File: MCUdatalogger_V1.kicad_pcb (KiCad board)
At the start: 2 copper layers, 29 parts, among them J1 Conn_01x04_Pin, J2 Conn_01x04_Pin, J3 Conn_01x09_Pin, J4 Conn_02x03_Odd_Even, U1 24LC1025, U2 DS1337S+, U3 24LC1025, U4 ATMEGA328P-AU, Y1 32.768 KHz, Y2 16 MHz

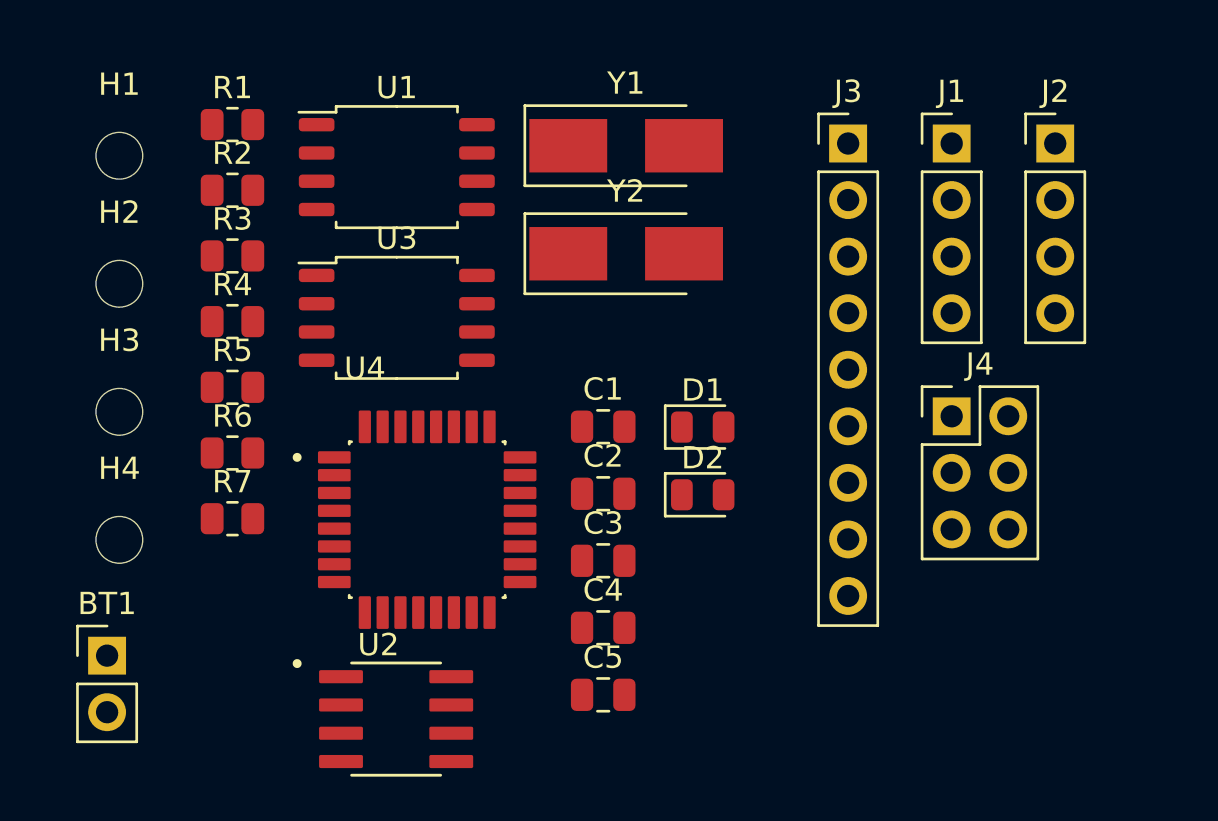
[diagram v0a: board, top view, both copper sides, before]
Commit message: Connections established
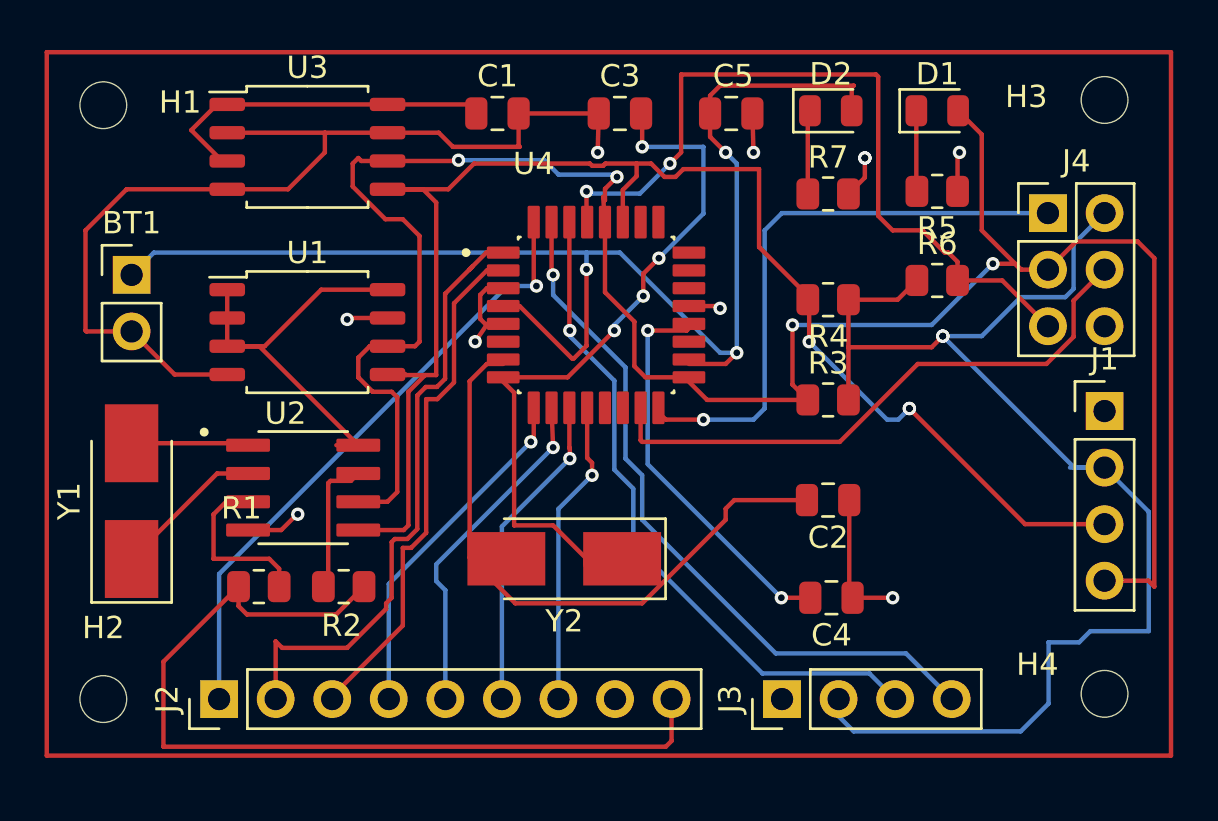
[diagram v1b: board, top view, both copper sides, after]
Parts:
- moved H3 46.4 mm to (123.7, 46.8)
- moved H4 44.8 mm to (123.7, 73.4)
- moved J2 37.7 mm to (83.9, 73.7), turned to 90 degrees
- moved R5 32.9 mm to (116.2, 50.9), turned to 180 degrees
- moved R6 32.6 mm to (116.2, 54.9)
- moved R7 30.5 mm to (111.3, 51.0)
- moved J3 27.8 mm to (109.2, 73.7), turned to 90 degrees
- moved R3 27.5 mm to (111.3, 60.2)
- moved Y1 27.3 mm to (80.0, 64.8), turned to 90 degrees
- moved R4 26.8 mm to (111.3, 55.7), turned to 180 degrees
- moved C5 26.7 mm to (106.9, 47.4)
- moved R1 20.8 mm to (85.7, 68.6)
- moved C3 20.1 mm to (101.9, 47.4)
- moved H2 18.7 mm to (78.7, 73.7)
- moved R2 18.5 mm to (89.5, 68.6), turned to 180 degrees
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- renumbered J3 to J2, J2 to J3
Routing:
- net /VCC: track 0.00 -> 137.1 mm, vias 0 -> 2
- net /SCK: track 0.00 -> 100.2 mm, vias 0 -> 4
- net /SDA: track 0.00 -> 68.1 mm, vias 0 -> 3
- net GND: track 0.00 -> 67.0 mm, vias 0 -> 10
- net Net-(BT1-+): track 0.00 -> 60.8 mm, vias 0 -> 3
- net /RESET: track 0.00 -> 35.5 mm, vias 0 -> 2
- net /TX: track 0.00 -> 32.1 mm, vias 0 -> 1
- net Net-(U4-PB7): track 0.00 -> 30.8 mm, vias 0 -> 4
- net /RX: track 0.00 -> 30.1 mm, vias 0 -> 1
- net /D2: track 0.00 -> 28.1 mm, vias 0 -> 1
- net Net-(U4-PB6): track 0.00 -> 28.0 mm
- net /D3: track 0.00 -> 27.8 mm
- net /MISO: track 0.00 -> 26.4 mm, vias 0 -> 1
- net /MOSI: track 0.00 -> 26.3 mm
- net /D4: track 0.00 -> 23.4 mm
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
